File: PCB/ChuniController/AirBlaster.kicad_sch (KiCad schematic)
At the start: 1 part, among them J8 Conn_01x08

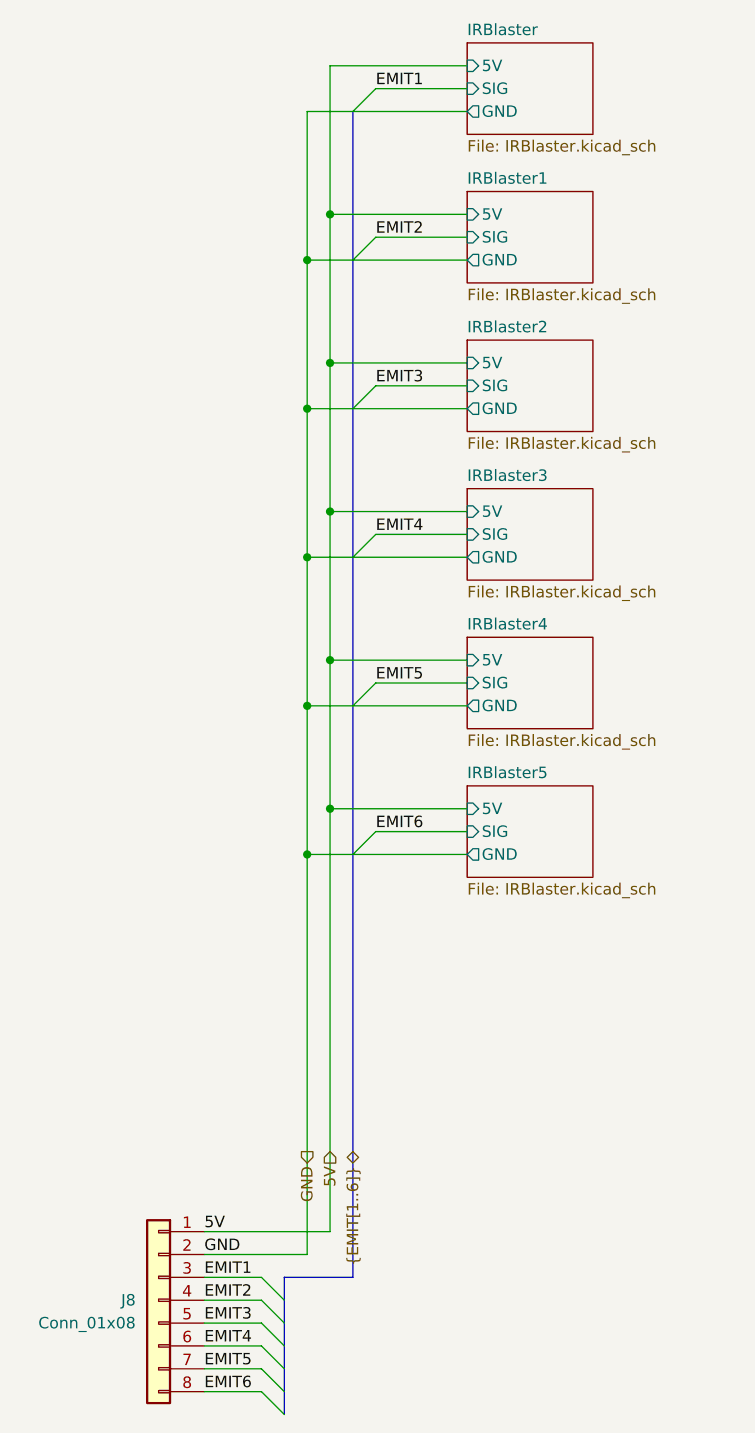
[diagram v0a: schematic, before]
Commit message: PCB
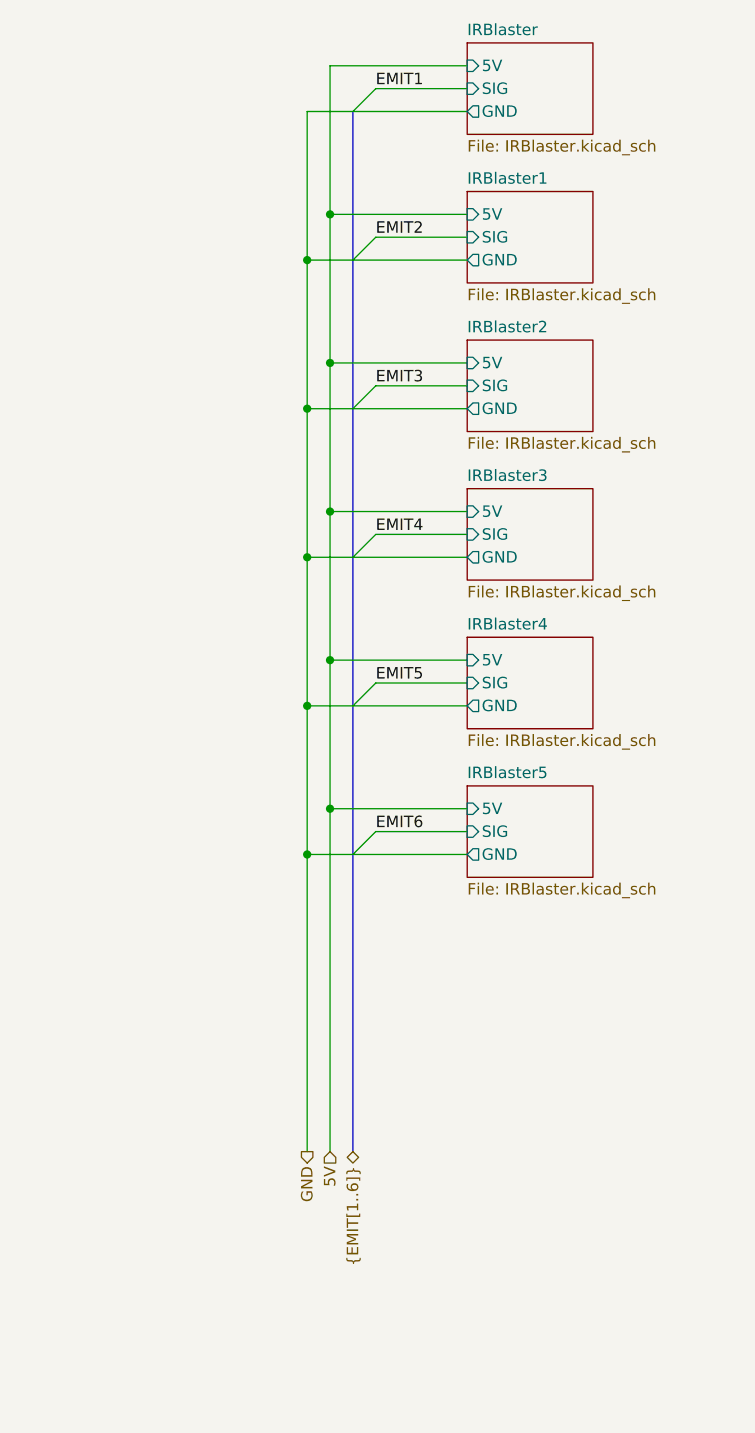
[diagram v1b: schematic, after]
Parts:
- removed J8: Conn_01x08, Connector_JST:JST_SH_SM08B-SRSS-TB_1x08-1MP_P1.00mm_Horizontal, symbol Connector_Generic:Conn_01x08
